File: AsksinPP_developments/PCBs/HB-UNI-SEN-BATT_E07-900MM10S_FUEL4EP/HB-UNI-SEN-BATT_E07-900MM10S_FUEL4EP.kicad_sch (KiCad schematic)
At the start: 32 parts, among them J1 Conn_01x02, J10 charge, J11 ePaper connector, J12 U.FL connector, J2 Conn_01x02, J3 Conn_01x02, J4 Conn_01x02, J5 ISP Programmer, J6 Conn_01x04, J7 Conn_01x04, J8 Conn_01x04, J9 Conn_01x04, Q1 IRLU024N, SW1 config button

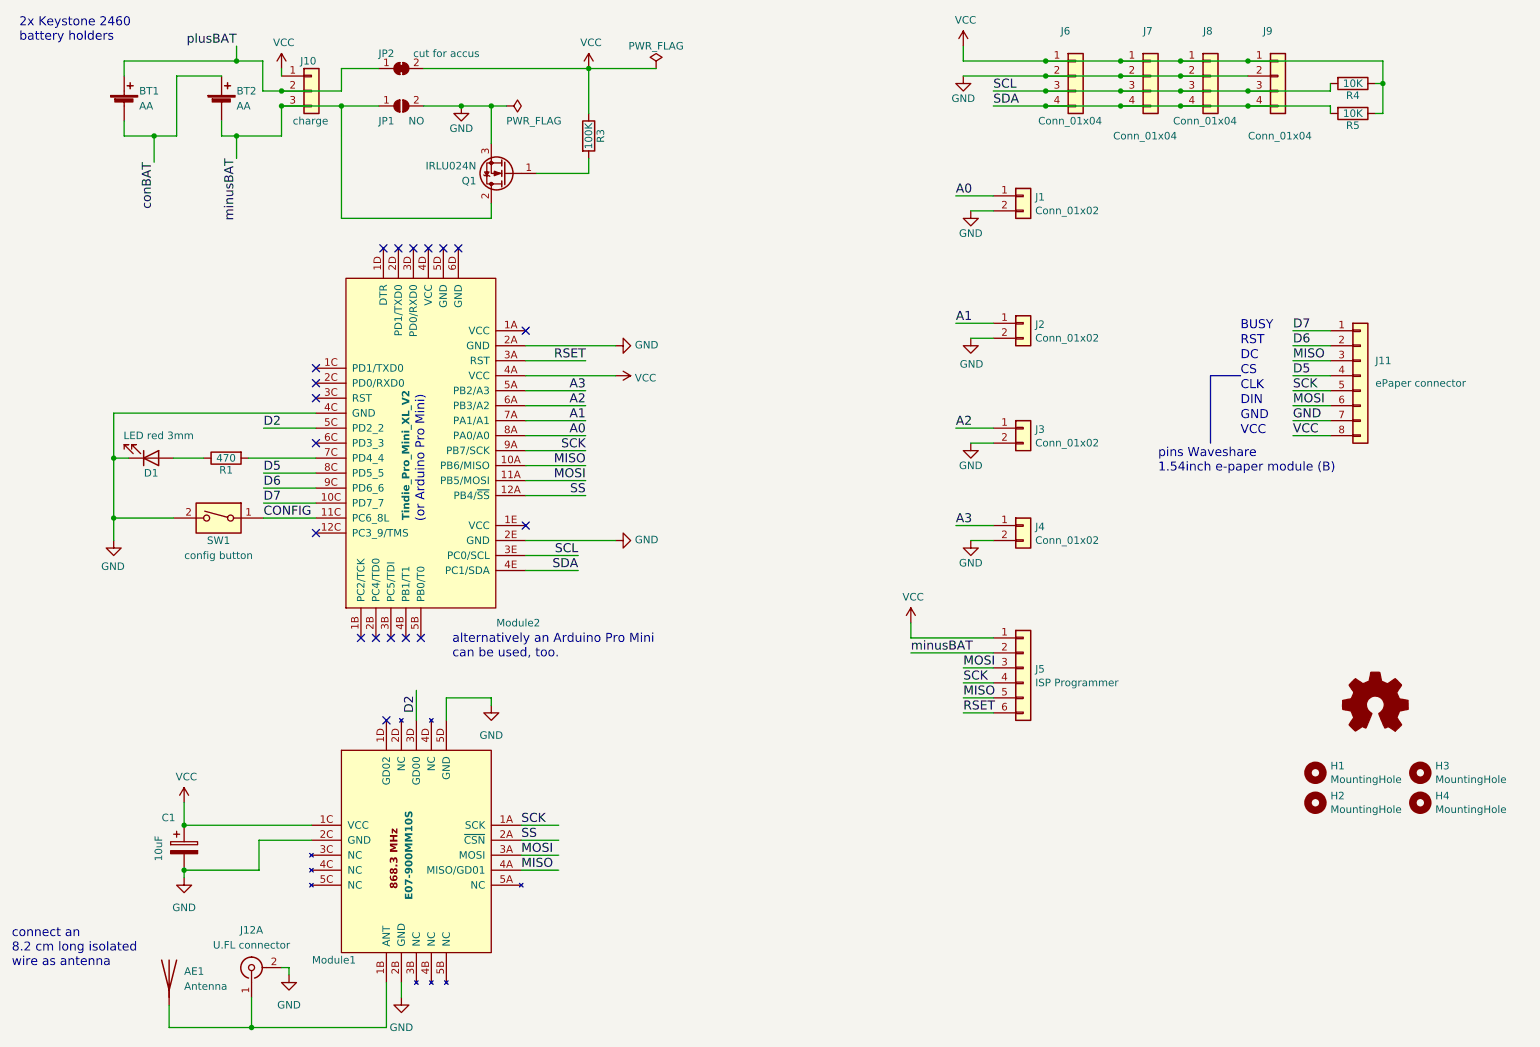
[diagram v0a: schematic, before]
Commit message: PCBs/HB-UNI-SEN-BATT_E07-900MM10S_FUEL4EP: migration to KiCAD 8
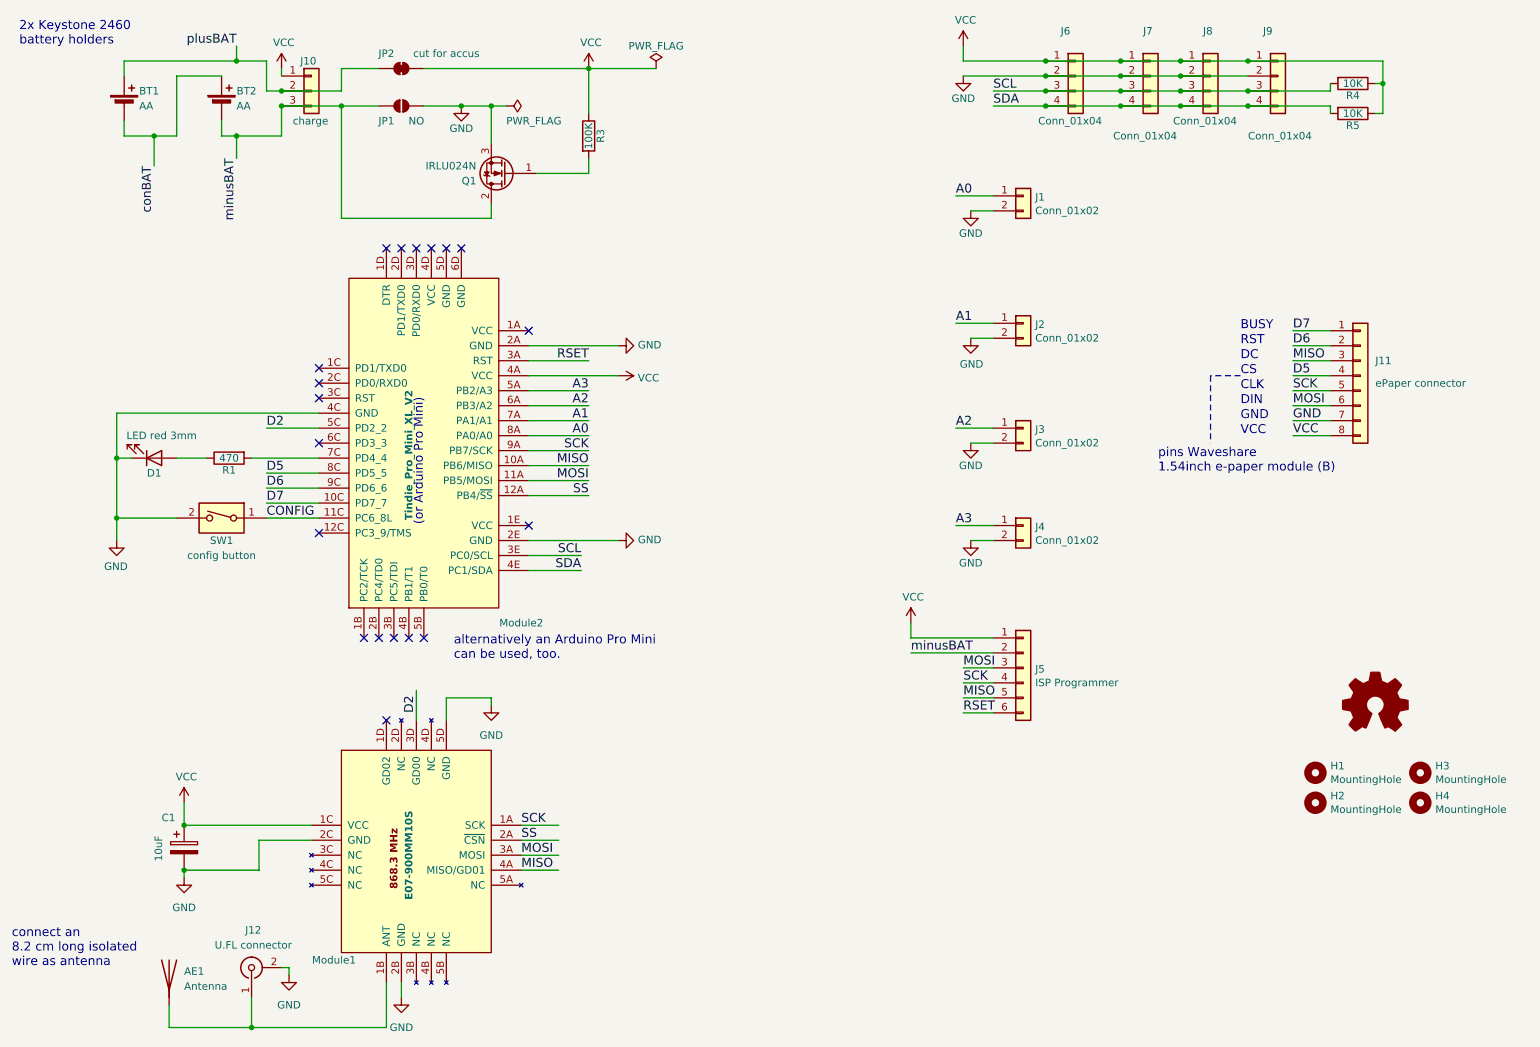
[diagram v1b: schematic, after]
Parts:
- removed J12: U.FL connector, FUEL4EP:U.FL_Molex_MCRF_73412-0110_Vertical, symbol Connector:Conn_Coaxial_x2_Isolated
- added J12: U.FL connector, FUEL4EP:U.FL_Molex_MCRF_73412-0110_Vertical, symbol Connector:Conn_Coaxial
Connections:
- net GND: now also J12.2 (Ext)
- net at AE1.1 (A), Module1.1B (ANT): now also J12.1 (In)
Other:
- moved on the sheet: D1, Module2, R1, SW1
